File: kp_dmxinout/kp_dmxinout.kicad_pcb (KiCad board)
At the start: 2 copper layers, 9 parts, among them J1 NC3MAAH, J2 NC3FAAH, J3 Conn_01x04, U1 SN75176AD, U2 6N137, U3 6N137, U4 SN75176AD

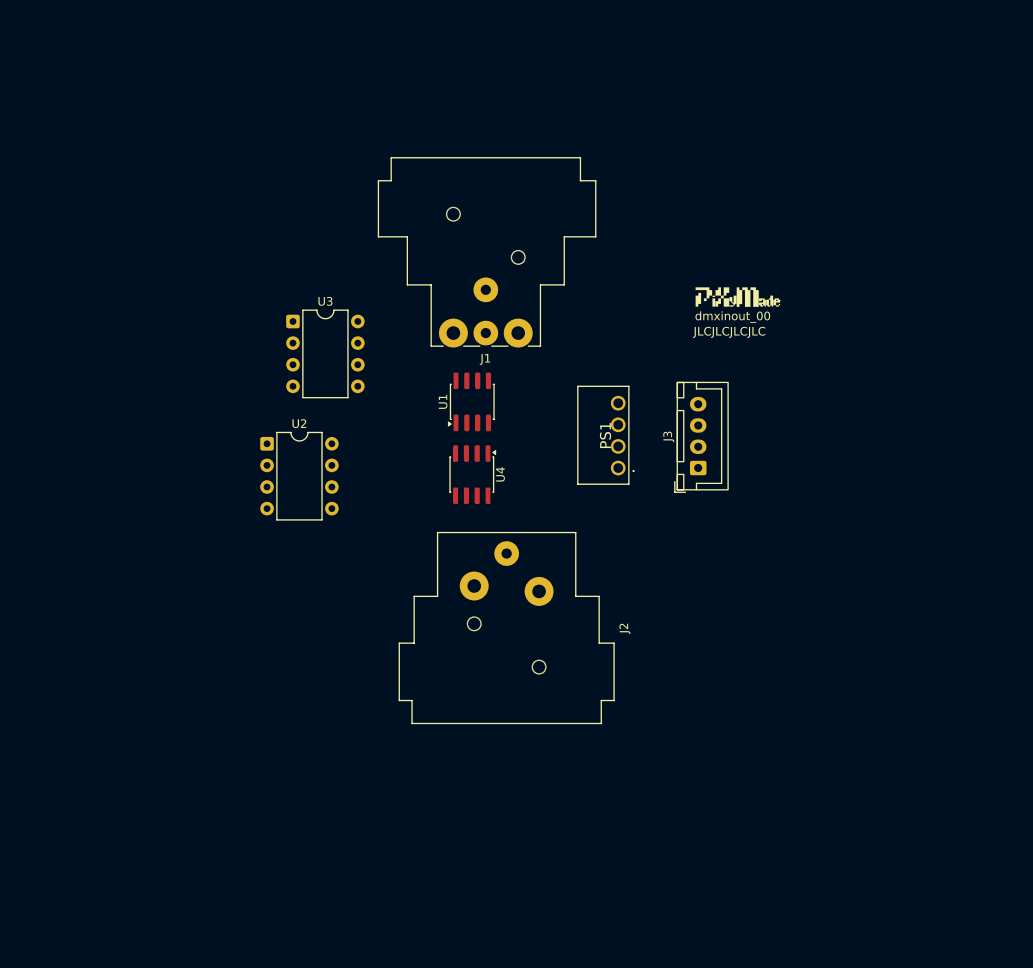
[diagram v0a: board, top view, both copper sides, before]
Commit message: dmxinout: do board
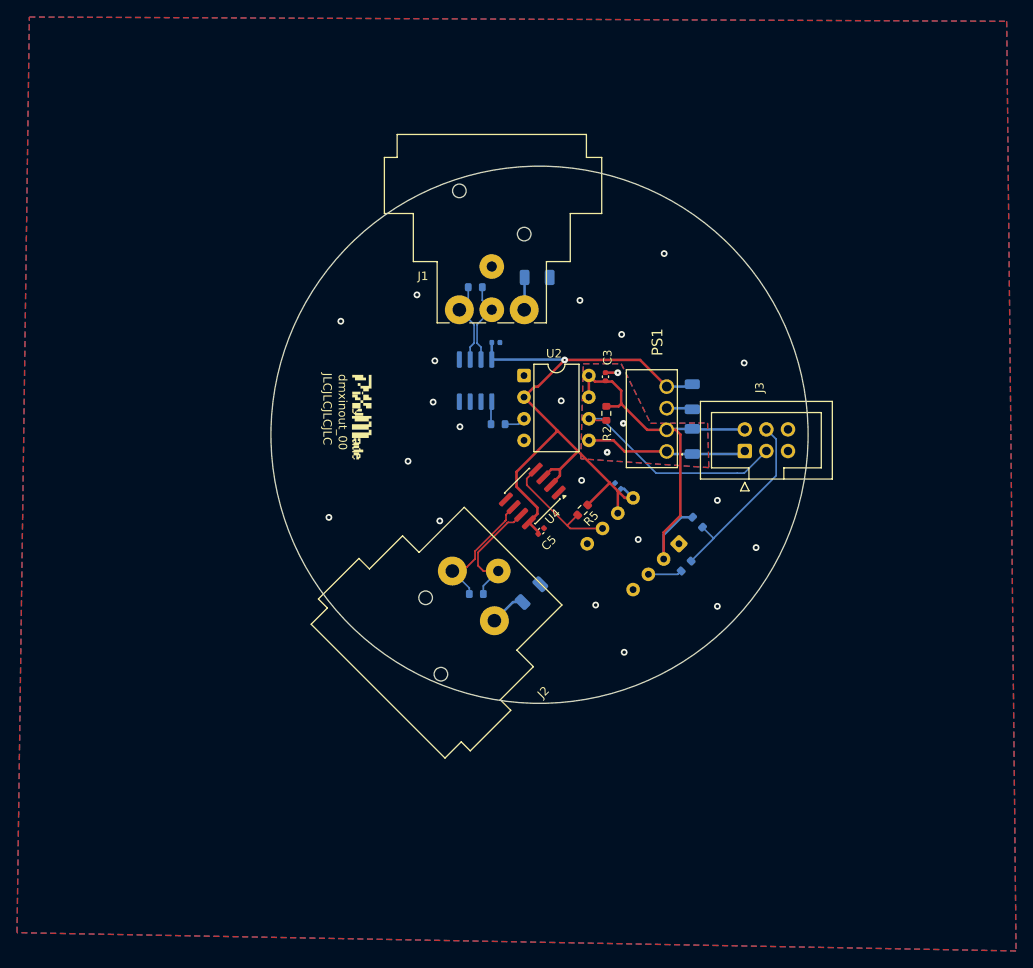
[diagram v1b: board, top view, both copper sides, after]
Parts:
- added C1: 4.7u, Capacitor_SMD:C_1206_3216Metric, B.Cu at (190.9, 66.9)
- added C2: 10u, Capacitor_SMD:C_1206_3216Metric, B.Cu at (190.9, 61.7)
- added C3: 100n, Capacitor_SMD:C_0402_1005Metric, F.Cu at (180.8, 59.3)
- added C4: 100n, Capacitor_SMD:C_0402_1005Metric, B.Cu at (167.9, 55.3)
- added C5: 100n, Capacitor_SMD:C_0402_1005Metric, F.Cu at (173.2, 77.5)
- added C6: 100n, Capacitor_SMD:C_0402_1005Metric, B.Cu at (182.2, 72.2)
- added C7: 1u, Capacitor_SMD:C_1206_3216Metric, B.Cu at (172.7, 47.6)
- added C8: 1u, Capacitor_SMD:C_1206_3216Metric, B.Cu at (172.1, 84.8)
- added R1: 470, Resistor_SMD:R_0603_1608Metric, B.Cu at (168.1, 64.9)
- added R2: 3000, Resistor_SMD:R_0603_1608Metric, F.Cu at (180.8, 63.6)
- added R3: 470, Resistor_SMD:R_0603_1608Metric, B.Cu at (190.2, 81.6)
- added R4: 3000, Resistor_SMD:R_0603_1608Metric, B.Cu at (191.6, 76.4)
- added R5: 3000, Resistor_SMD:R_0603_1608Metric, F.Cu at (178.1, 75.0)
- added R6: 120, Resistor_SMD:R_0603_1608Metric, B.Cu at (165.6, 84.8)
- added R7: 120, Resistor_SMD:R_0603_1608Metric, B.Cu at (165.4, 48.8)
- J3: footprint Connector_JST:JST_XH_B4B-XH-A_1x04_P2.50mm_Vertical -> Connector_IDC:IDC-Header_2x03_P2.54mm_Vertical
- U1, U3: moved to B.Cu
- moved U3 52.3 mm to (189.4, 78.9), turned to 135 degrees
- moved G*** 46.4 mm to (152.1, 64.1), turned to -90 degrees
- moved U2 31.2 mm to (171.2, 59.2)
- moved U4 7.54 mm to (172.1, 73.3), turned to -135 degrees
- moved J2 6.28 mm to (167.7, 88.0), turned to -135 degrees
- moved PS1 6.02 mm to (187.9, 68.1)
- moved J3 5.82 mm to (197.1, 68.0)
- moved J1 2.83 mm to (171.2, 51.5)
- moved U1 2.53 mm to (165.5, 59.8)
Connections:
- net IN_DATAMINUS renamed IN_DATA-
- net IN_DATAPLUS renamed IN_DATA+
- net OUT_DATAMINUS renamed OUT_DATA-
- net OUT_DATAPLUS renamed OUT_DATA+
- J1 pad 1: Earth -> IN_SHIELD
- J1 pad G: Earth -> unconnected-(J1-PadG)
- J2 pad 1: Earth -> OUT_SHIELD
- U2 pad 3: Net-(U2-C) -> /6n137_in_c
- U3 pad 3: Net-(U3-C) -> /6n137_out_c
- U3 pad 6: IN_DATATTL -> OUT_DATATTL
- U4 pad 4: IN_DATATTL -> OUT_DATATTL
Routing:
- net +5V: track 0.00 -> 83.2 mm, vias 0 -> 1
- net +5V_IN: track 0.00 -> 50.9 mm
- net MCU_DMX_IN: track 0.00 -> 26.7 mm
- net MCU_DMX_OUT: track 0.00 -> 22.0 mm
- net GND_IN: track 0.00 -> 20.6 mm, vias 0 -> 3
- net OUT_DATATTL: track 0.00 -> 15.0 mm
- net OUT_DATA+: track 0.00 -> 14.7 mm
- net OUT_DATA-: track 0.00 -> 14.5 mm
- net IN_DATA-: track 0.00 -> 9.87 mm
- net IN_DATA+: track 0.00 -> 9.84 mm
- net OUT_SHIELD: track 0.00 -> 4.22 mm
- net /6n137_out_c: track 0.00 -> 4.02 mm
- net IN_SHIELD: track 0.00 -> 3.82 mm
- net GND: track 0.00 -> 3.05 mm, vias 0 -> 20
- net IN_DATATTL: track 0.00 -> 2.69 mm
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- added copper zone on B.Cu, net GND
- added copper zone on F.Cu, net GND
- added copper zone on B.Cu, net GND_IN
- added copper zone on F.Cu, net GND_IN
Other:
- board outline added: 63.1 x 63.1 mm
